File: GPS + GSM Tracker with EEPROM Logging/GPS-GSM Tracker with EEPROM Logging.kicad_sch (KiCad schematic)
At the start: 55 parts, among them J1 SIM_Card, U1 ESP32-S3-WROOM-1, U10 MT3608, U2 NEO-8Q, U3 CAT24C256, U4 SIM800C, U5 TXS0108EPW, U6 AMS1117-5.0, U7 PAT1220-C-10DB, U8 PAT1220-C-10DB, U9 TP4056

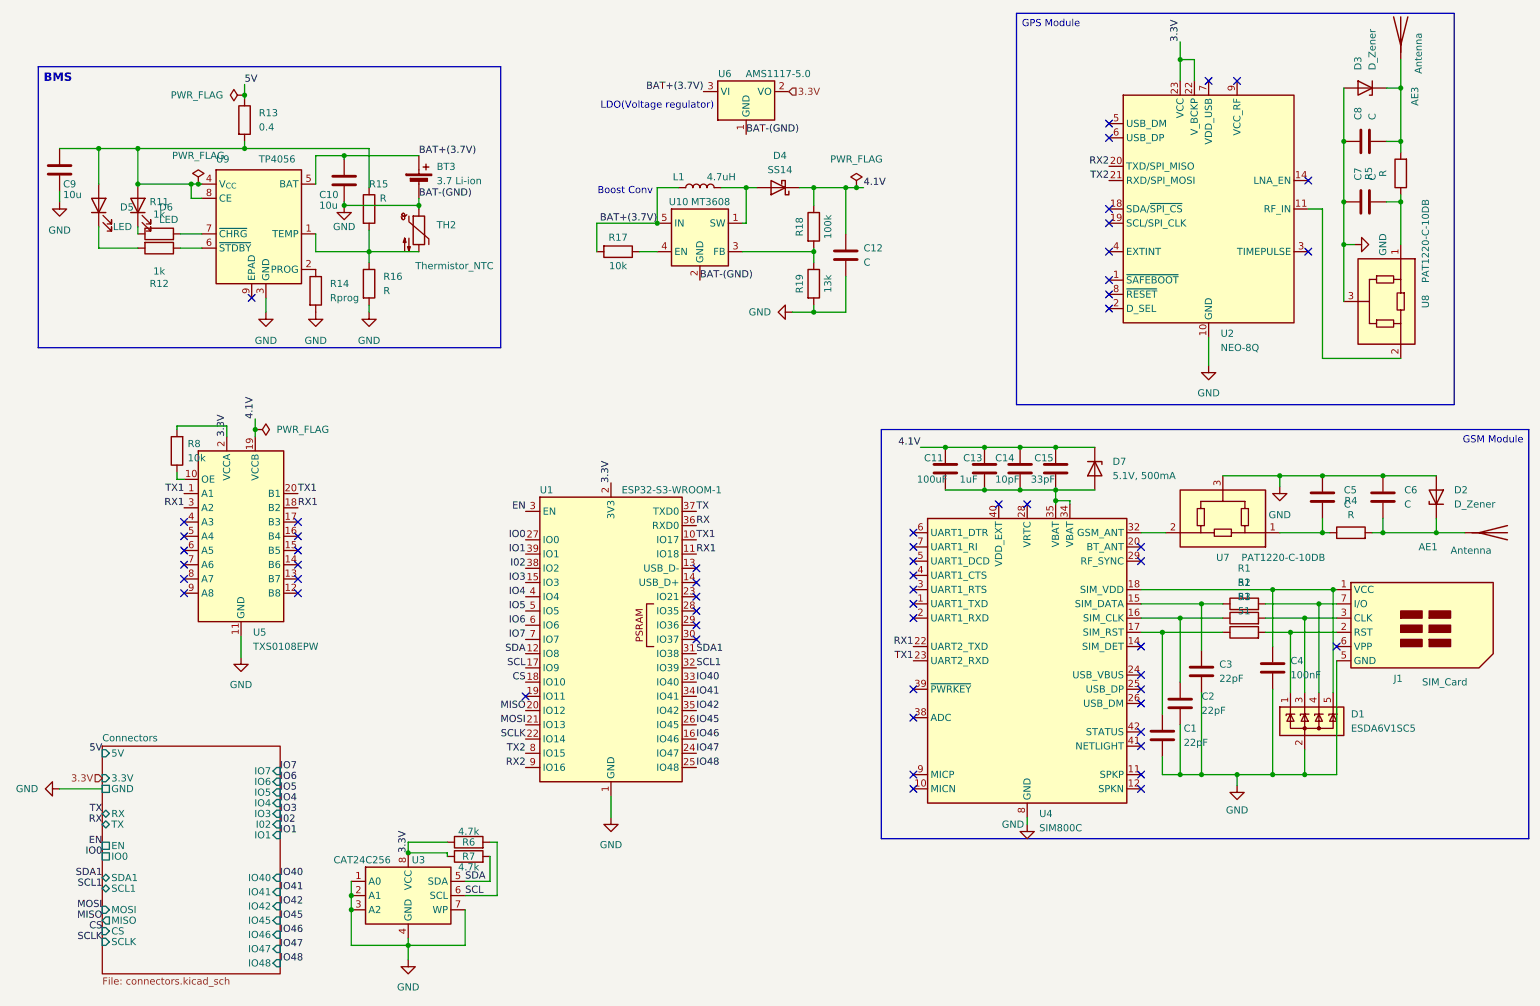
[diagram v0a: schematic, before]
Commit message: Completed Pcb design
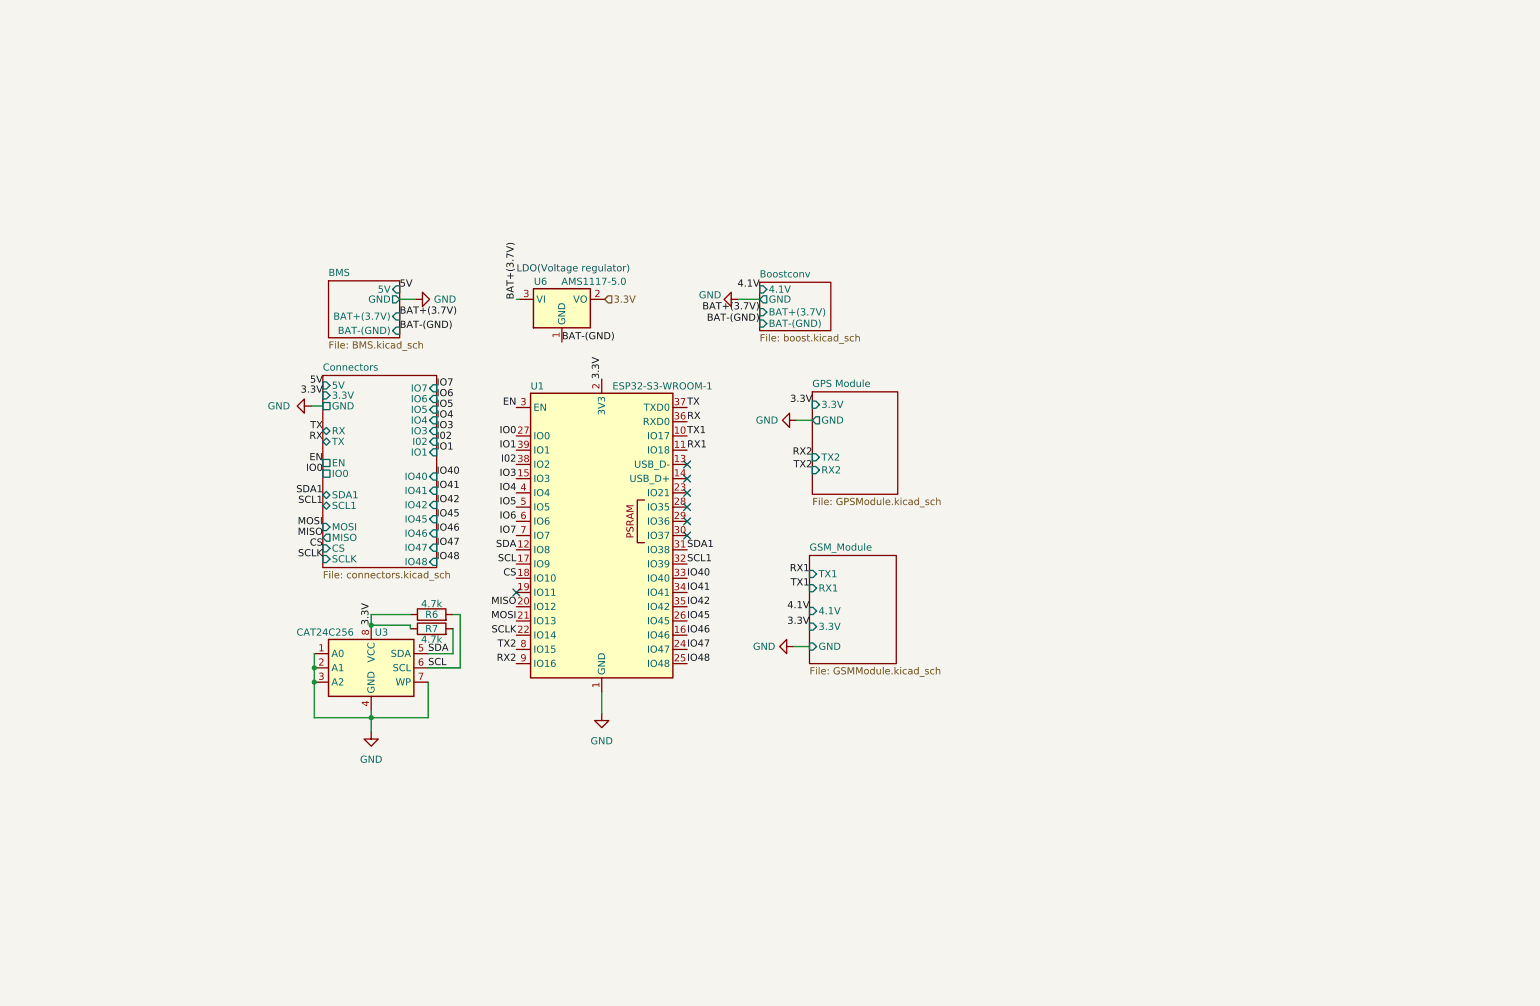
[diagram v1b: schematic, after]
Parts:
- removed AE1, AE3: Antenna, symbol Device:Antenna
- removed BT3: 3.7 Li-ion, symbol Device:Battery_Cell
- removed C1, C2, C3: 22pF, Capacitor_SMD:C_0805_2012Metric, symbol Device:C
- removed C10, C9: 10u, Capacitor_SMD:C_0805_2012Metric, symbol Device:C
- removed C11: 100uF, Capacitor_SMD:C_0805_2012Metric, symbol Device:C
- removed C12, C5, C6, C7, C8: C, Capacitor_SMD:C_0805_2012Metric, symbol Device:C
- removed C13: 1uF, Capacitor_SMD:C_0805_2012Metric, symbol Device:C
- removed C14: 10pF, Capacitor_SMD:C_0805_2012Metric, symbol Device:C
- removed C15: 33pF, Capacitor_SMD:C_0805_2012Metric, symbol Device:C
- removed C4: 100nF, Capacitor_SMD:C_0805_2012Metric, symbol Device:C
- removed D1: ESDA6V1SC5, Package_TO_SOT_SMD:SOT-23-5, symbol Power_Protection:ESDA6V1SC5
- removed D2, D3: D_Zener, symbol Device:D_Zener
- removed D4: SS14, Diode_SMD:D_SMA, symbol Diode:SS14
- removed D5, D6: LED, LED_SMD:LED_0805_2012Metric, symbol Device:LED
- removed D7: 5.1V, 500mA, symbol Device:D_Zener
- removed J1: SIM_Card, symbol Connector:SIM_Card
- removed L1: 4.7uH, Inductor_SMD:L_0805_2012Metric, symbol Device:L
- removed R1, R2, R3: 51, Resistor_SMD:R_0805_2012Metric, symbol Device:R
- removed R11, R12: 1k, Resistor_SMD:R_0805_2012Metric, symbol Device:R
- removed R13: 0.4, Resistor_SMD:R_0805_2012Metric, symbol Device:R
- removed R14: Rprog, Resistor_SMD:R_0805_2012Metric, symbol Device:R
- removed R15, R16, R4, R5: R, Resistor_SMD:R_0805_2012Metric, symbol Device:R
- removed R17, R8: 10k, Resistor_SMD:R_0805_2012Metric, symbol Device:R
- removed R18: 100k, Resistor_SMD:R_0805_2012Metric, symbol Device:R
- removed R19: 13k, Resistor_SMD:R_0805_2012Metric, symbol Device:R
- removed TH2: Thermistor_NTC, symbol Device:Thermistor_NTC
- removed U10: MT3608, Package_TO_SOT_SMD:SOT-23-6, symbol Regulator_Switching:MT3608
- removed U2: NEO-8Q, RF_GPS:ublox_NEO, symbol RF_GPS:NEO-8Q
- removed U4: SIM800C, RF_GSM:SIMCom_SIM800C, symbol RF_GSM:SIM800C
- removed U5: TXS0108EPW, Package_SO:TSSOP-20_4.4x6.5mm_P0.65mm, symbol Logic_LevelTranslator:TXS0108EPW
- removed U7, U8: PAT1220-C-10DB, RF_Converter:RF_Attenuator_Susumu_PAT1220, symbol RF:PAT1220-C-10DB
- removed U9: TP4056, Package_SO:SOIC-8-1EP_3.9x4.9mm_P1.27mm_EP2.41x3.3mm_ThermalVias, symbol Battery_Management:TP4056-42-ESOP8
- U3: footprint (none) -> Package_SO:SOIC-8_3.9x4.9mm_P1.27mm
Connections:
- net GND: no longer U6.1 (GND)
- new net BAT-(GND): U6.1 (GND)
- no-connect marks 56 -> 7
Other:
- added sheet BMS (BMS.kicad_sch)
- added sheet Boostconv (boost.kicad_sch)
- added sheet GPS Module (GPSModule.kicad_sch)
- added sheet GSM_Module (GSMModule.kicad_sch)
- note removed: "Boost Conv"
- moved on the sheet: R6, R7, U1, U3, U6
